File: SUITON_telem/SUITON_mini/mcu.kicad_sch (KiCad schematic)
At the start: 27 parts, among them J1 USB_C_Receptacle_USB2.0_14P, J2 Conn_01x06_Pin, U12 STM32H743VIT6, X1 ABM3B-8.000MHZ-10-1UT

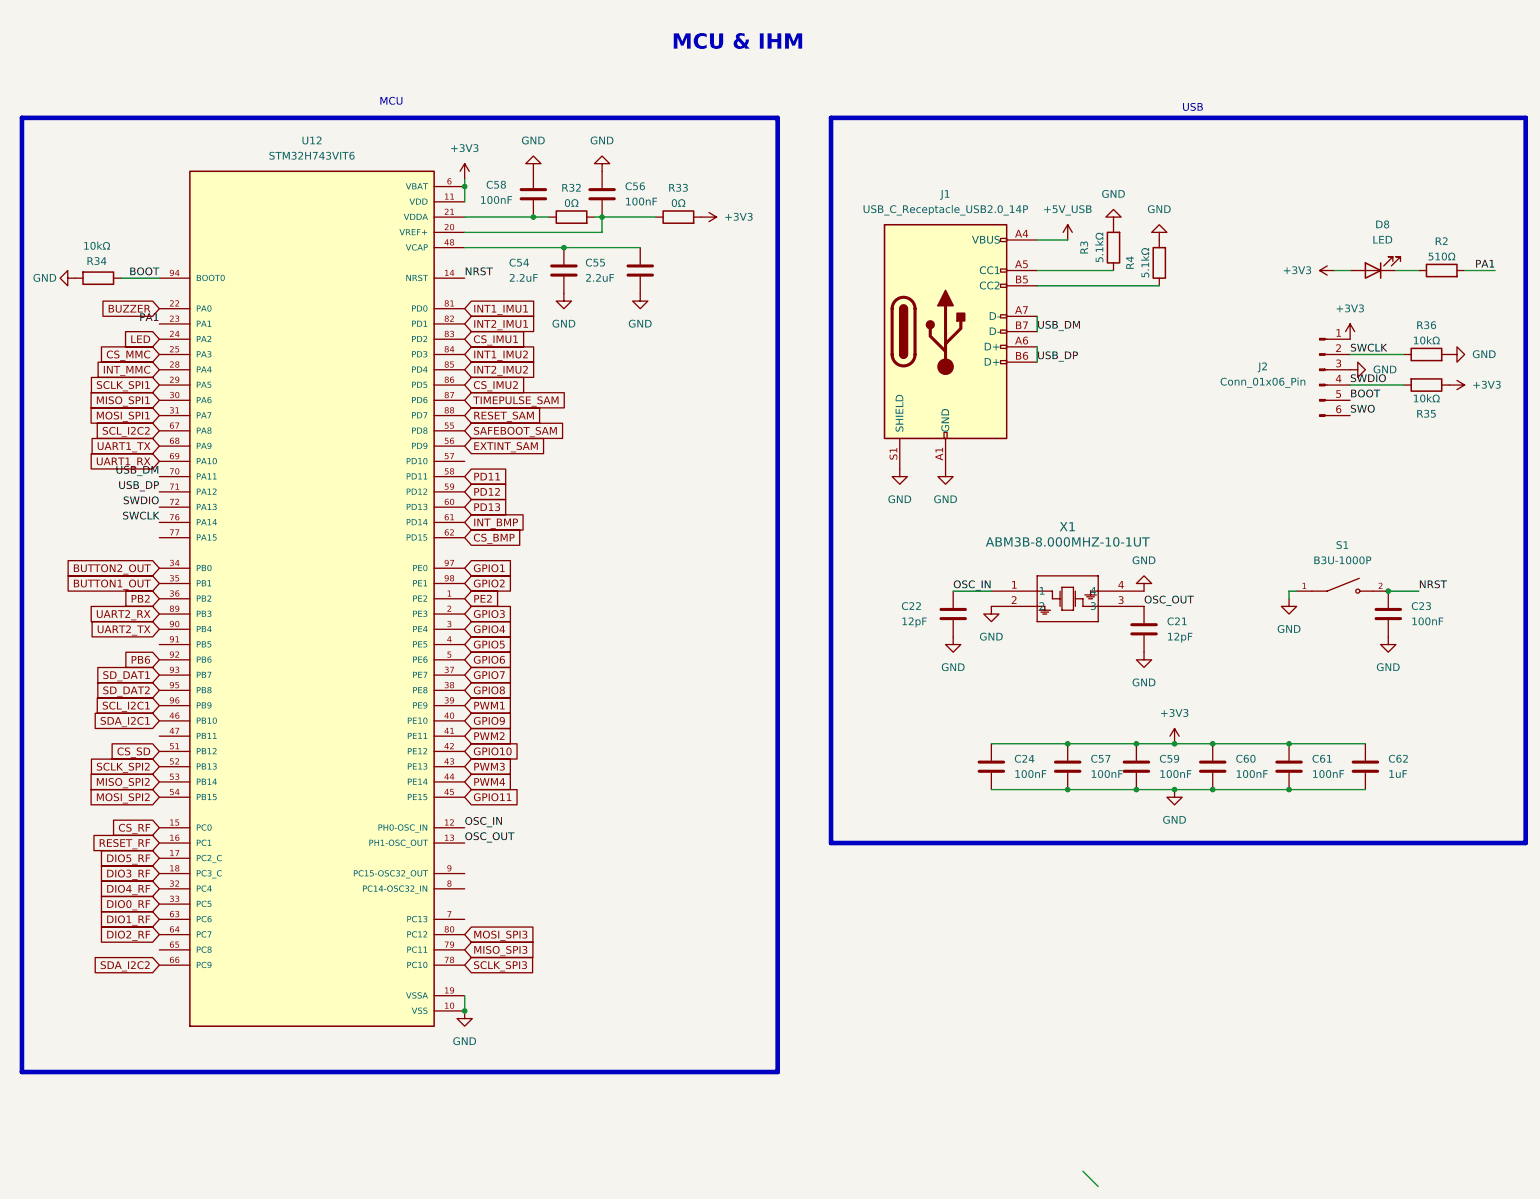
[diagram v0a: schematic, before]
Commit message: SUITON mini
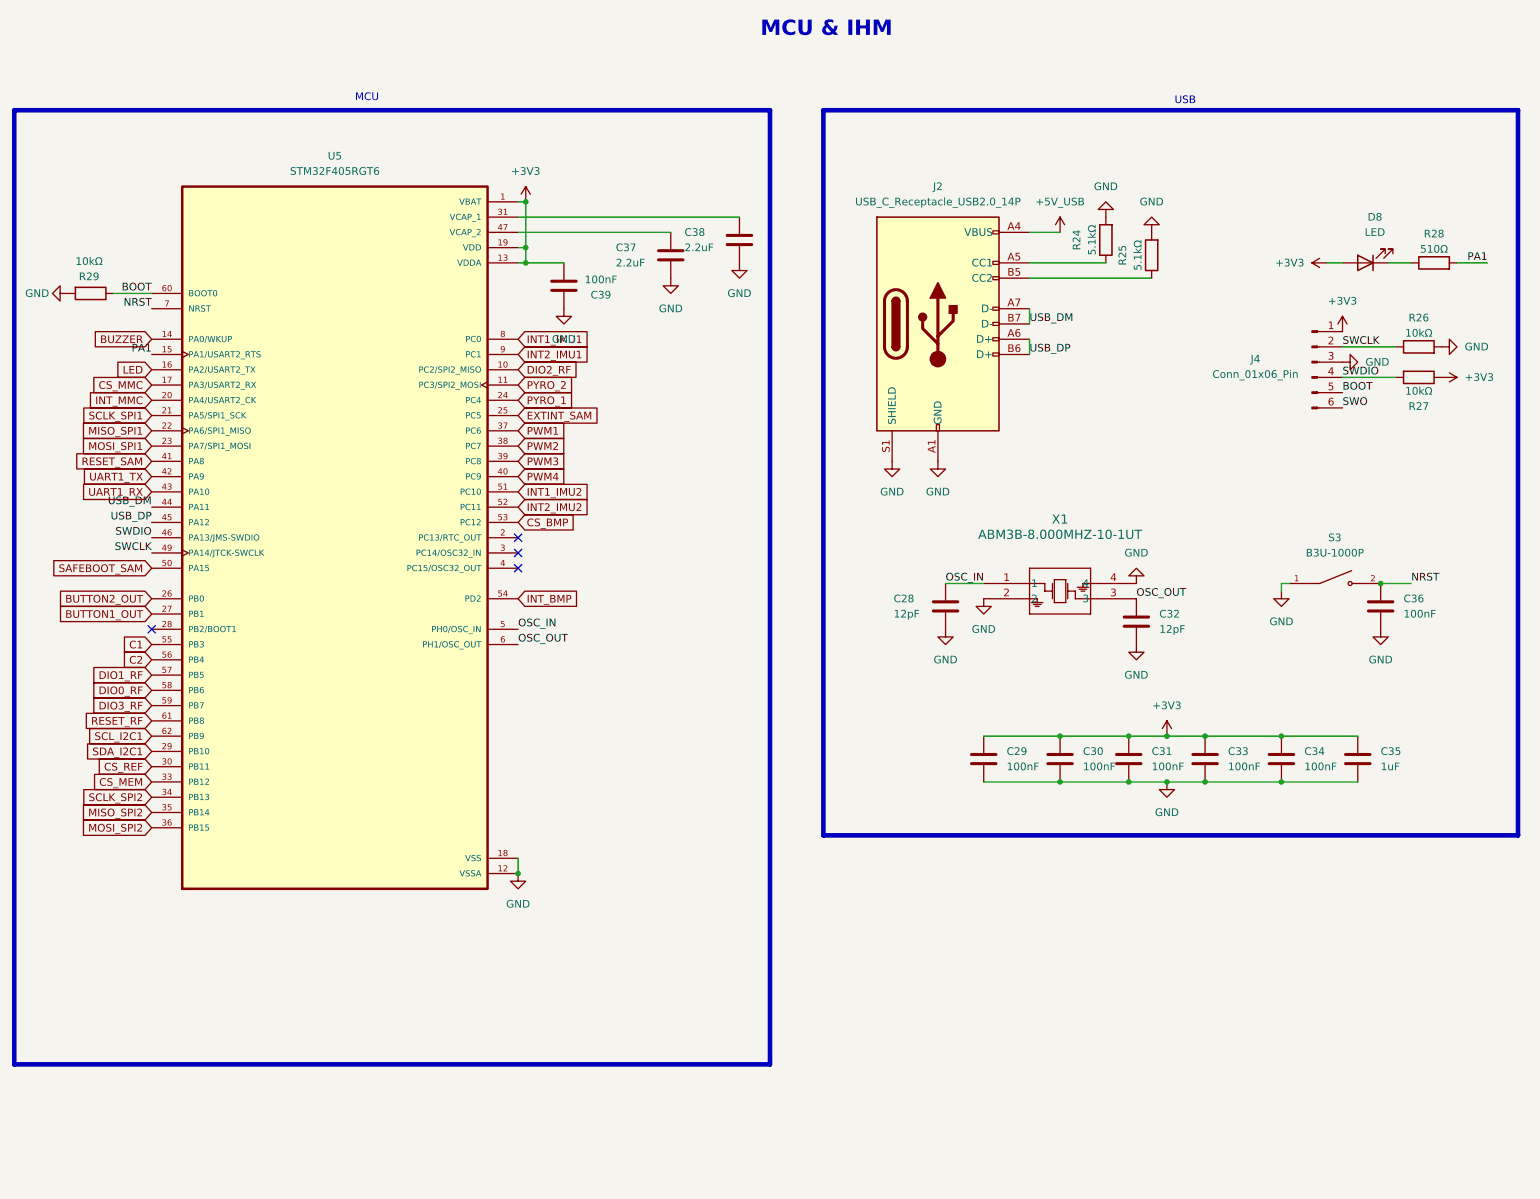
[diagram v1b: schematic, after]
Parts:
- removed C21, C22: 12pF, Capacitor_SMD:C_0603_1608Metric, symbol Device:C
- removed C23, C24, C56, C57, C58, C59, C60, C61: 100nF, Capacitor_SMD:C_0603_1608Metric, symbol Device:C
- removed C54, C55: 2.2uF, symbol Device:C
- removed C62: 1uF, Capacitor_SMD:C_0603_1608Metric, symbol Device:C
- removed J1: USB_C_Receptacle_USB2.0_14P, symbol Connector:USB_C_Receptacle_USB2.0_14P
- removed J2: Conn_01x06_Pin, symbol Connector:Conn_01x06_Pin
- removed R2: 510Ω, symbol Device:R
- removed R3, R4: 5.1kΩ, symbol Device:R
- removed R32, R33: 0Ω, symbol Device:R
- removed R34, R35, R36: 10kΩ, symbol Device:R
- removed S1: B3U-1000P, B3U-1000P:SW_B3U-1000P, symbol B3U-1000P:B3U-1000P
- removed U12: STM32H743VIT6, STM32H743VIT6:QFP50P1600X1600X160-100N, symbol STM32H743VIT6:STM32H743VIT6
- added C28, C32: 12pF, Capacitor_SMD:C_0603_1608Metric, symbol Device:C
- added C29, C30, C31, C33, C34, C36, C39: 100nF, Capacitor_SMD:C_0603_1608Metric, symbol Device:C
- added C35: 1uF, Capacitor_SMD:C_0603_1608Metric, symbol Device:C
- added C37, C38: 2.2uF, symbol Device:C
- added J2: USB_C_Receptacle_USB2.0_14P, symbol Connector:USB_C_Receptacle_USB2.0_14P
- added J4: Conn_01x06_Pin, symbol Connector:Conn_01x06_Pin
- added R24, R25: 5.1kΩ, symbol Device:R
- added R26, R27, R29: 10kΩ, symbol Device:R
- added R28: 510Ω, symbol Device:R
- added S3: B3U-1000P, B3U-1000P:SW_B3U-1000P, symbol B3U-1000P:B3U-1000P
- added U5: STM32F405RGT6, STM32F405RGT6:QFP50P1200X1200X160-64N, symbol STM32F405RGT6:STM32F405RGT6
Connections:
- net +3V3: now also C29.1, C30.1, C31.1, C33.1, C34.1, C35.1, C39.2, J4.1 (Pin_1), R27.1, U5.1 (VBAT), U5.13 (VDDA), U5.19 (VDD), U5.32 (VDD), U5.48 (VDD), U5.64 (VDD)
- net +5V_USB: now also J2.A4 (VBUS), J2.A9 (VBUS), J2.B4 (VBUS), J2.B9 (VBUS)
- net BOOT: now also J4.5 (Pin_5), R29.1, U5.60 (BOOT0)
- net BUTTON1_OUT: now also U5.27 (PB1)
- net BUTTON2_OUT: now also U5.26 (PB0)
- net BUZZER: now also U5.14 (PA0/WKUP)
- net CS_BMP: now also U5.53 (PC12)
- net CS_MMC: now also U5.17 (PA3/USART2_RX)
- net DIO0_RF: now also U5.58 (PB6)
- net DIO1_RF: now also U5.57 (PB5)
- net DIO2_RF: now also U5.10 (PC2/SPI2_MISO)
- net DIO3_RF: now also U5.59 (PB7)
- net EXTINT_SAM: now also U5.25 (PC5)
- net GND: now also C28.2, C29.2, C30.2, C31.2, C32.2, C33.2, C34.2, C35.2, C36.2, C37.2, C38.2, C39.1, J2.A1 (GND), J2.A12 (GND), J2.B1 (GND), J2.B12 (GND), J2.S1 (SHIELD), J4.3 (Pin_3), R24.2, R25.2, R26.2, R29.2, S3.1, U5.12 (VSSA), U5.18 (VSS), U5.63 (VSS)
- net INT1_IMU1: now also U5.8 (PC0)
- net INT1_IMU2: now also U5.51 (PC10)
- net INT2_IMU1: now also U5.9 (PC1)
- net INT2_IMU2: now also U5.52 (PC11)
- net INT_BMP: now also U5.54 (PD2)
- net INT_MMC: now also U5.20 (PA4/USART2_CK)
- net LED: now also U5.16 (PA2/USART2_TX)
- net MISO_SPI1: now also U5.22 (PA6/SPI1_MISO)
- net MISO_SPI2: now also U5.35 (PB14)
- net MOSI_SPI1: now also U5.23 (PA7/SPI1_MOSI)
- net MOSI_SPI2: now also U5.36 (PB15)
- net NRST: now also C36.1, S3.2, U5.7 (NRST)
- net OSC_IN: now also C28.1, U5.5 (PH0/OSC_IN)
- net OSC_OUT: now also C32.1, U5.6 (PH1/OSC_OUT)
- net PA1: now also R28.2, U5.15 (PA1/USART2_RTS)
- net PWM1: now also U5.37 (PC6)
- net PWM2: now also U5.38 (PC7)
- net PWM3: now also U5.39 (PC8)
- net PWM4: now also U5.40 (PC9)
- net RESET_RF: now also U5.61 (PB8)
- net RESET_SAM: now also U5.41 (PA8)
- net SAFEBOOT_SAM: now also U5.50 (PA15)
- net SCLK_SPI1: now also U5.21 (PA5/SPI1_SCK)
- net SCLK_SPI2: now also U5.34 (PB13)
- net SCL_I2C1: now also U5.62 (PB9)
- net SDA_I2C1: now also U5.29 (PB10)
- net SWCLK: now also J4.2 (Pin_2), R26.1, U5.49 (PA14/JTCK-SWCLK)
- net SWDIO: now also J4.4 (Pin_4), R27.2, U5.46 (PA13/JMS-SWDIO)
- net SWO: now also J4.6 (Pin_6)
- net UART1_RX: now also U5.43 (PA10)
- net UART1_TX: now also U5.42 (PA9)
- net USB_DM: now also J2.A7 (D-), J2.B7 (D-), U5.44 (PA11)
- net USB_DP: now also J2.A6 (D+), J2.B6 (D+), U5.45 (PA12)
- net at D8.1 (K): now also R28.1
- new net: C38.1, U5.31 (VCAP_1)
- new net: C37.1, U5.47 (VCAP_2)
- new net: J2.A5 (CC1), R24.1
- new net: J2.B5 (CC2), R25.1
- new net C1: U5.55 (PB3)
- new net C2: U5.56 (PB4)
- new net CS_MEM: U5.33 (PB12)
- new net CS_REF: U5.30 (PB11)
- new net PYRO_1: U5.24 (PC4)
- new net PYRO_2: U5.11 (PC3/SPI2_MOSI)
- no-connect marks 0 -> 4
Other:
- title: SUITON PRO -> SUITON mini

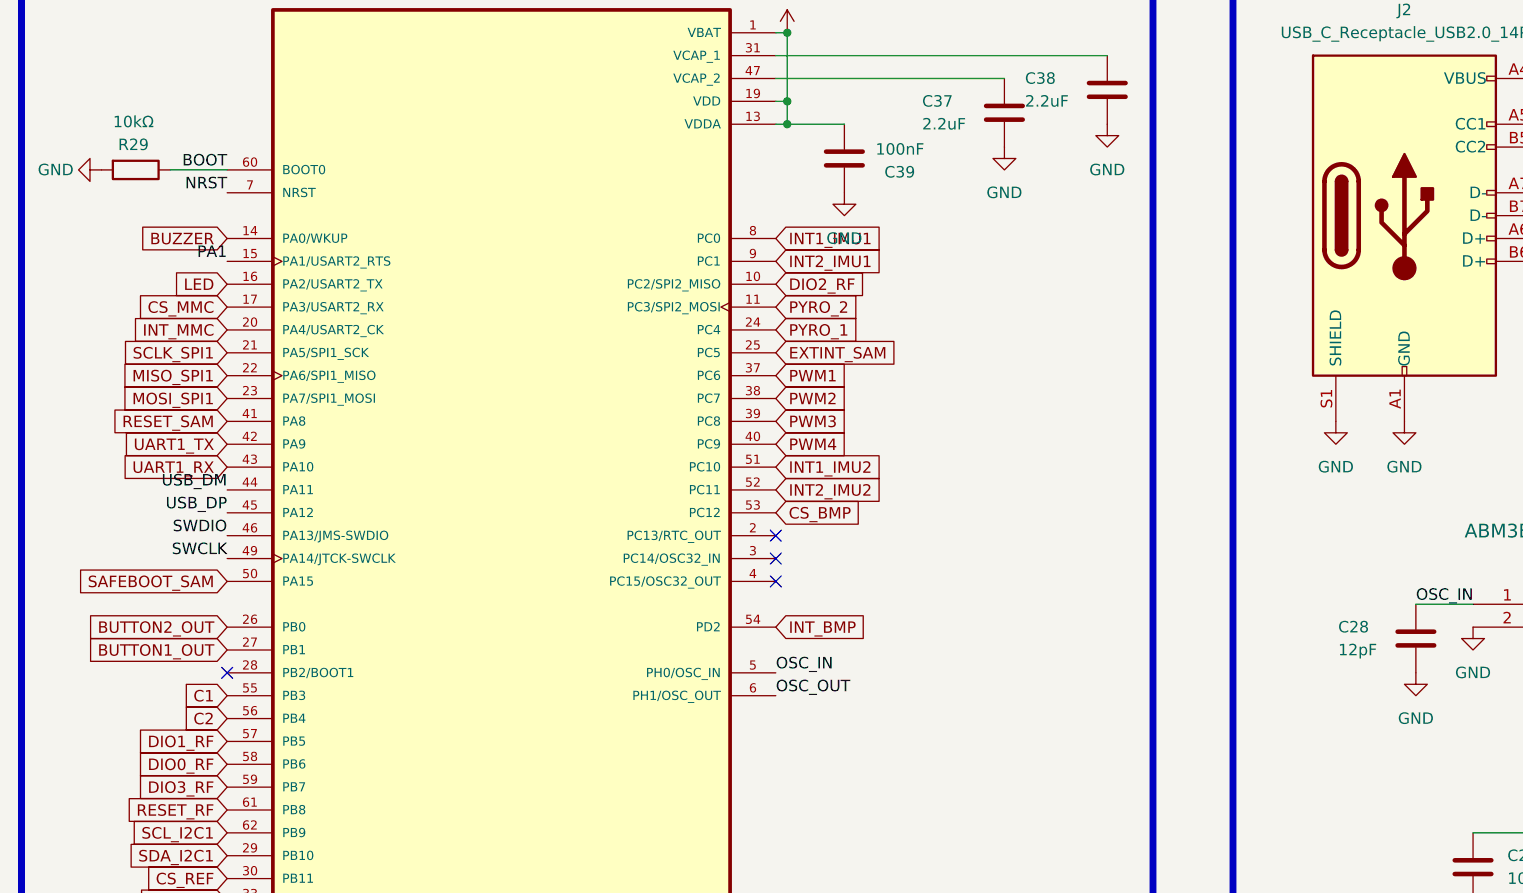
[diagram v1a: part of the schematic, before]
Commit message: New rf module
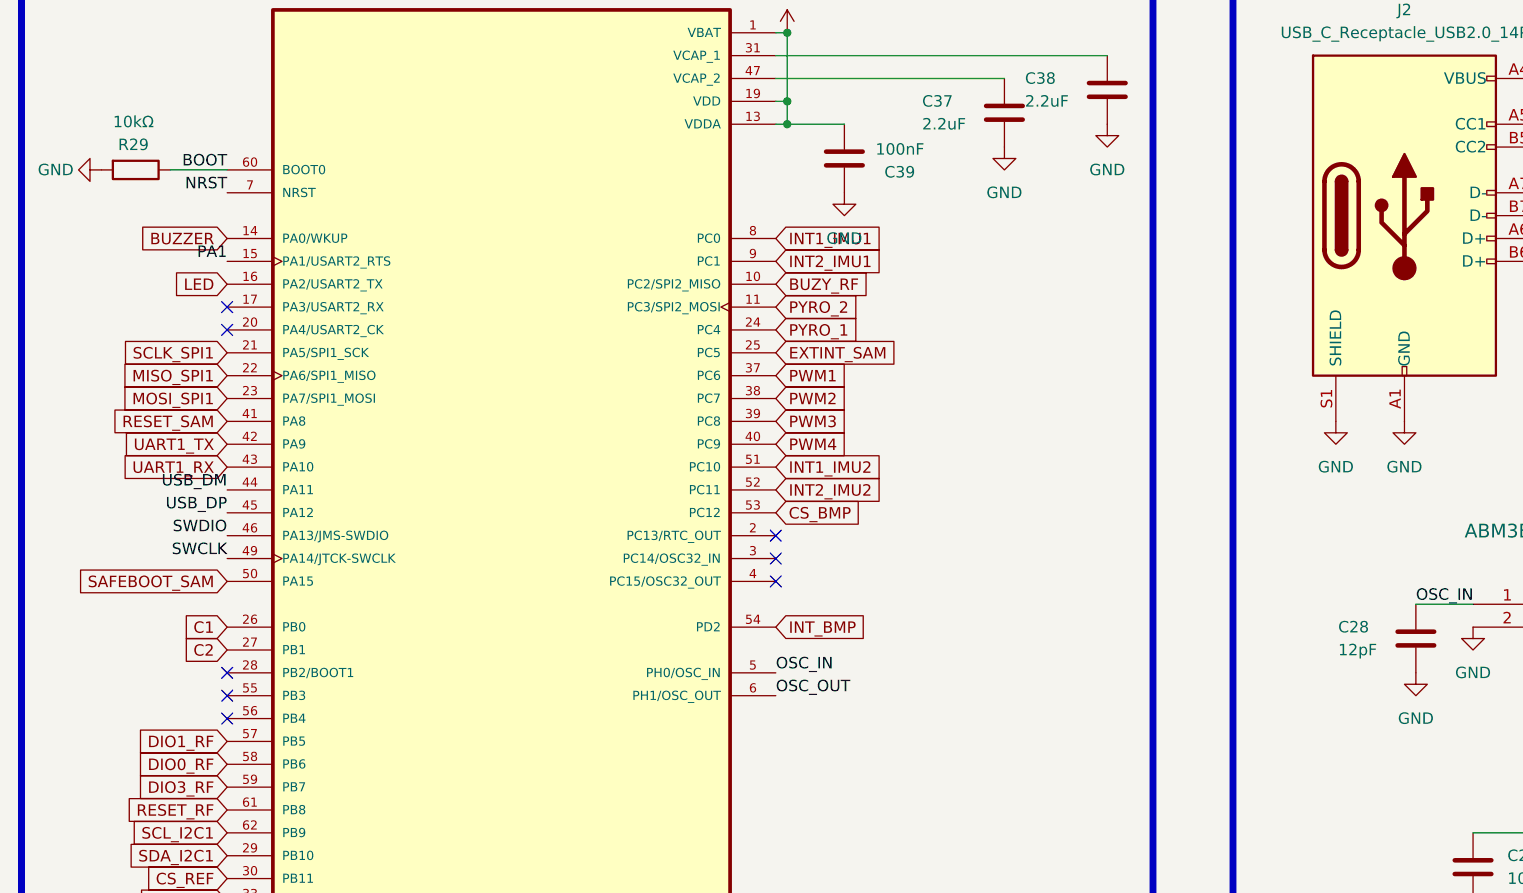
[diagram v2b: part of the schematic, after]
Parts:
- S3: DESCRIPTION Tactile Switch SPST-NO Top Actuated Surface Mount -> (none)
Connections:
- net BUTTON1_OUT is gone; now on net C2: U5.27 (PB1)
- net BUTTON2_OUT is gone; now on net C1: U5.26 (PB0)
- net C1: no longer U5.55 (PB3)
- net C2: no longer U5.56 (PB4)
- net CS_MMC: no longer names the net of U5.17 (PA3/USART2_RX)
- net DIO2_RF renamed BUZY_RF
- net INT_MMC: no longer names the net of U5.20 (PA4/USART2_CK)
- no-connect marks 4 -> 8
